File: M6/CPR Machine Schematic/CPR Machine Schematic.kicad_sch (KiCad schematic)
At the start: 0 parts

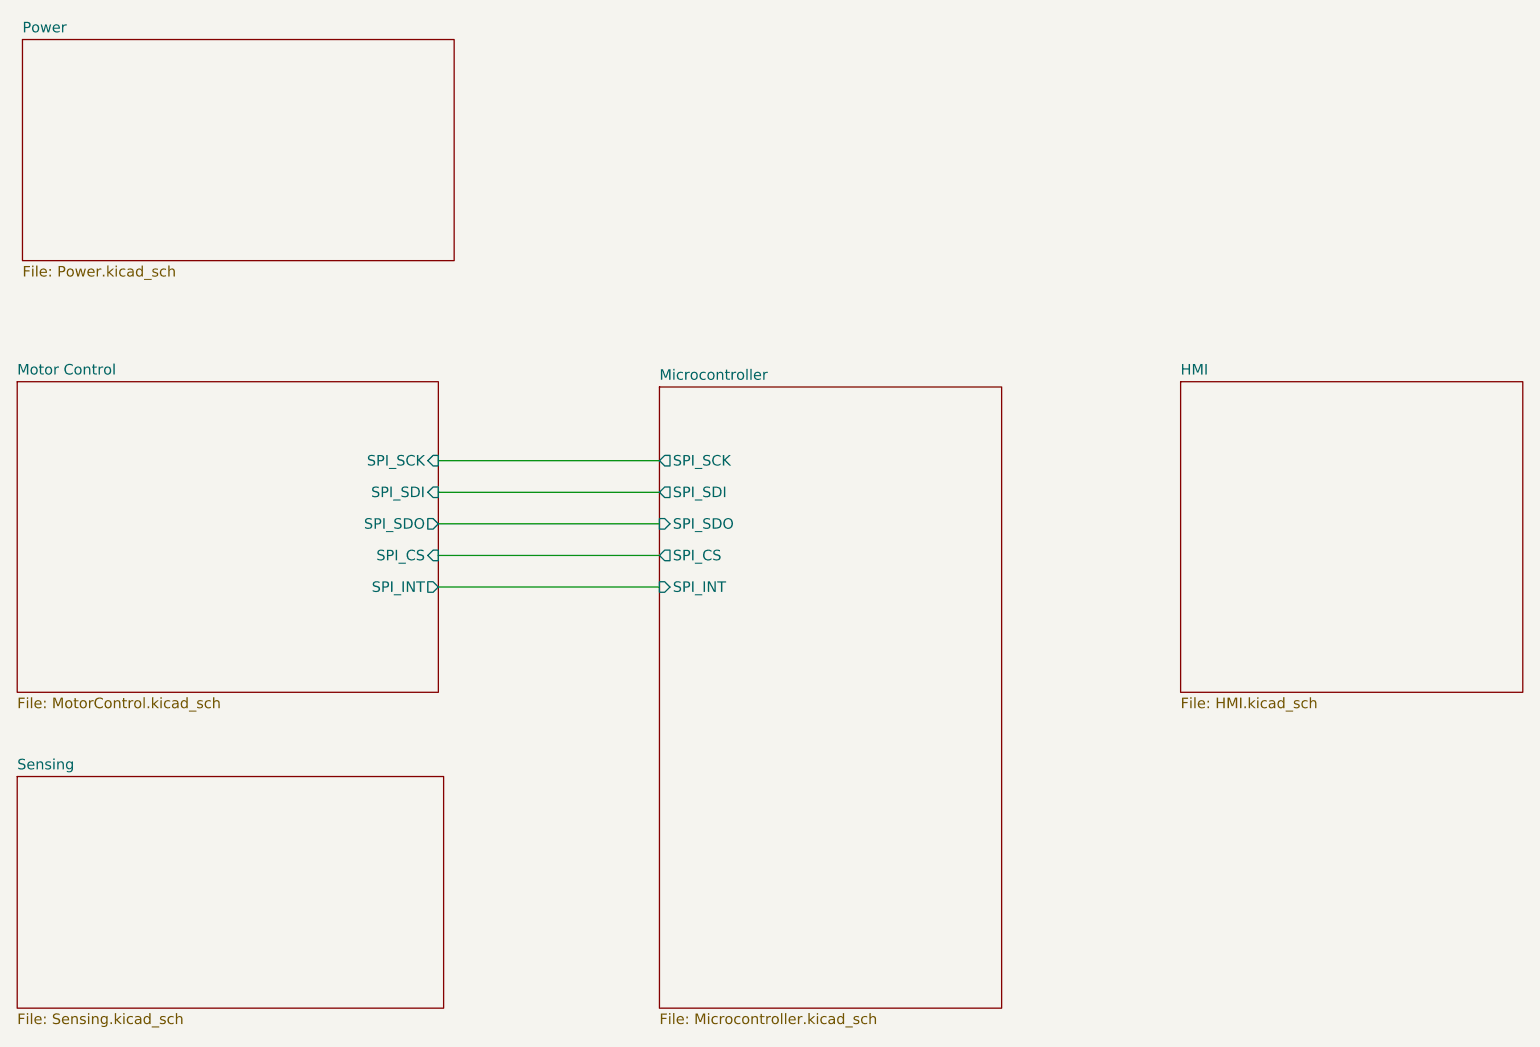
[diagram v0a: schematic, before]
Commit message: morer kicad
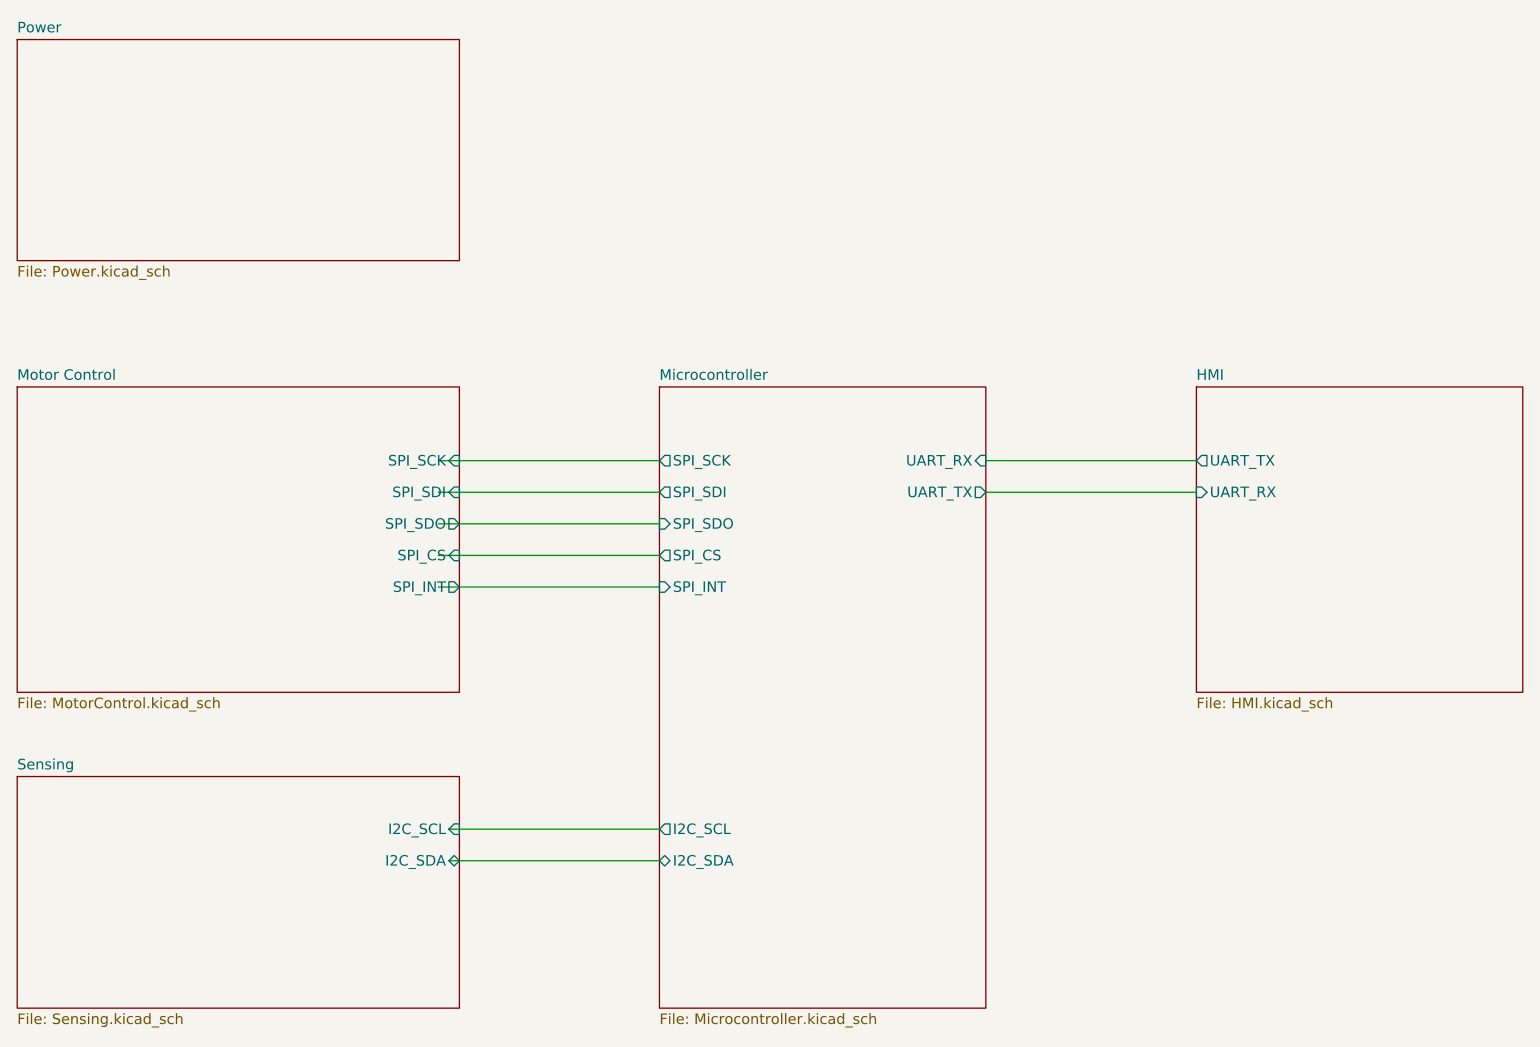
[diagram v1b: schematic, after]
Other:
- sheet HMI ports: added UART_RX, UART_TX; removed none
- sheet Microcontroller ports: added I2C_SCL, I2C_SDA, UART_RX, UART_TX; removed none
- sheet Sensing ports: added I2C_SCL, I2C_SDA; removed none
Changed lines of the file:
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@@
+	(wire
+		(pts
+			(xy 152.4 87.63) (xy 177.8 87.63)
+		)
+		(stroke
+			(width 0)
+			(type default)
+		)
+	)
 	(wire
 		(pts
@@
 	(wire
 		(pts
+			(xy 87.63 132.08) (xy 113.03 132.08)
+		)
+		(stroke
+			(width 0)
+			(type default)
+		)
+	)
+	(wire
+		(pts
+			(xy 87.63 135.89) (xy 113.03 135.89)
+		)
+		(stroke
+			(width 0)
+			(type default)
+		)
+	)
+	(wire
+		(pts
 			(xy 86.36 99.06) (xy 113.03 99.06)
 		)
@@
 		(pts
 			(xy 86.36 91.44) (xy 113.03 91.44)
+		)
+		(stroke
+			(width 0)
+			(type default)
+		)
+	)
+	(wire
+		(pts
+			(xy 152.4 91.44) (xy 177.8 91.44)
 		)
 		(stroke
@@
 	(sheet
 		(at 35.56 125.73)
-		(size 51.435 27.94)
+		(size 53.34 27.94)
 		(exclude_from_sim no)
 		(in_bom yes)
@@
 			)
 		)
+		(pin "I2C_SCL" input
+			(at 88.9 132.08 0)
+			(effects
+				(font
+					(size 1.27 1.27)
+				)
+				(justify right)
+			)
+		)
+		(pin "I2C_SDA" bidirectional
+			(at 88.9 135.89 0)
+			(effects
+				(font
+					(size 1.27 1.27)
+				)
+				(justify right)
+			)
+		)
 		(instances
 			(project "CPR Machine Schematic"
@@
 	)
 	(sheet
-		(at 36.195 36.83)
-		(size 52.07 26.67)
+		(at 35.56 36.83)
+		(size 53.34 26.67)
 		(exclude_from_sim no)
 		(in_bom yes)
@@
 		)
 		(property "Sheetname" "Power"
-			(at 36.195 36.1184 0)
+			(at 35.56 36.1184 0)
 			(effects
 				(font
@@
 		)
 		(property "Sheetfile" "Power.kicad_sch"
-			(at 36.195 64.0846 0)
+			(at 35.56 64.0846 0)
 			(effects
 				(font
@@
 	)
 	(sheet
-		(at 35.56 78.105)
-		(size 50.8 37.465)
+		(at 35.56 78.74)
+		(size 53.34 36.83)
 		(exclude_from_sim no)
 		(in_bom yes)
@@
 		)
 		(property "Sheetname" "Motor Control"
-			(at 35.56 77.3934 0)
+			(at 35.56 78.0284 0)
 			(effects
 				(font
@@
 		)
 		(pin "SPI_SCK" input
-			(at 86.36 87.63 0)
+			(at 88.9 87.63 0)
 			(effects
 				(font
@@
 		)
 		(pin "SPI_SDI" input
-			(at 86.36 91.44 0)
+			(at 88.9 91.44 0)
 			(effects
 				(font
@@
 		)
 		(pin "SPI_SDO" output
-			(at 86.36 95.25 0)
+			(at 88.9 95.25 0)
 			(effects
 				(font
@@
 		)
 		(pin "SPI_CS" input
-			(at 86.36 99.06 0)
+			(at 88.9 99.06 0)
 			(effects
 				(font
@@
 		)
 		(pin "SPI_INT" output
-			(at 86.36 102.87 0)
+			(at 88.9 102.87 0)
 			(effects
 				(font
@@
 	)
 	(sheet
-		(at 175.895 78.105)
-		(size 41.275 37.465)
+		(at 177.8 78.74)
+		(size 39.37 36.83)
 		(exclude_from_sim no)
 		(in_bom yes)
@@
 		)
 		(property "Sheetname" "HMI"
-			(at 175.895 77.3934 0)
+			(at 177.8 78.0284 0)
 			(effects
 				(font
@@
 		)
 		(property "Sheetfile" "HMI.kicad_sch"
-			(at 175.895 116.1546 0)
+			(at 177.8 116.1546 0)
 			(effects
 				(font
@@
 				)
 				(justify left top)
+			)
+		)
+		(pin "UART_RX" input
+			(at 177.8 91.44 180)
+			(effects
+				(font
+					(size 1.27 1.27)
+				)
+				(justify left)
+			)
+		)
+		(pin "UART_TX" output
+			(at 177.8 87.63 180)
+			(effects
+				(font
+					(size 1.27 1.27)
+				)
+				(justify left)
 			)
 		)
@@
 	(sheet
 		(at 113.03 78.74)
-		(size 41.275 74.93)
+		(size 39.37 74.93)
 		(exclude_from_sim no)
 		(in_bom yes)
@@
 			)
 		)
+		(pin "I2C_SDA" bidirectional
+			(at 113.03 135.89 180)
+			(effects
+				(font
+					(size 1.27 1.27)
+				)
+				(justify left)
+			)
+		)
+		(pin "I2C_SCL" output
+			(at 113.03 132.08 180)
+			(effects
+				(font
+					(size 1.27 1.27)
+				)
+				(justify left)
+			)
+		)
+		(pin "UART_TX" output
+			(at 152.4 91.44 0)
+			(effects
+				(font
+					(size 1.27 1.27)
+				)
+				(justify right)
+			)
+		)
+		(pin "UART_RX" input
+			(at 152.4 87.63 0)
+			(effects
+				(font
+					(size 1.27 1.27)
+				)
+				(justify right)
+			)
+		)
